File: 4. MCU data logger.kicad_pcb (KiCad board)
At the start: 2 copper layers, 50.2 x 30.3 mm, 29 parts, among them J1 Conn_01x04_Pin, J2 Conn_01x04_Pin, J3 Conn_01x09_Pin, J4 Conn_02x03_Odd_Even, U1 24LC1025, U2 24LC1025, U4 ATMEGA328P-AU, U5 DS1337S_, Y1 32.768 KHz, Y2 16 MHz

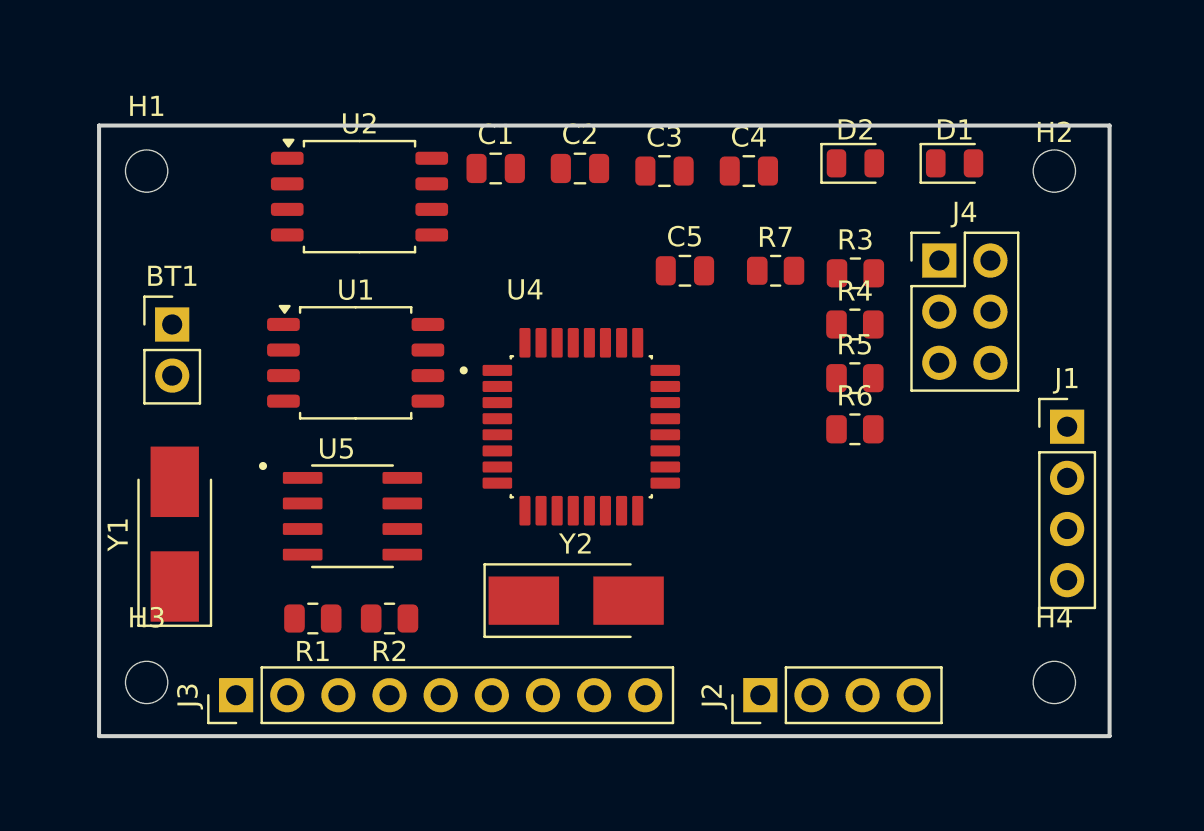
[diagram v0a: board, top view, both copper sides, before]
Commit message: Routing Completed
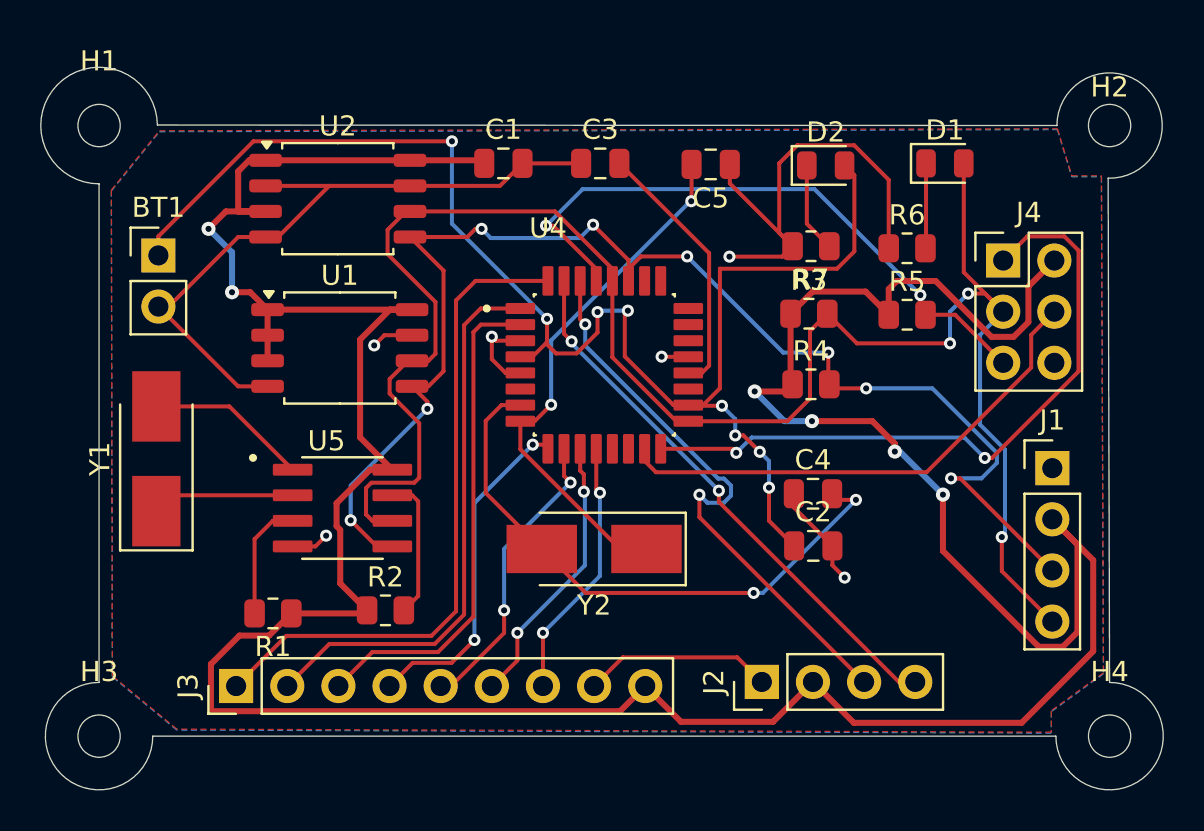
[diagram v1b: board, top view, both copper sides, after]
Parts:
- moved C2 22.0 mm to (80.7, 80.2)
- moved C4 16.3 mm to (80.7, 77.6)
- moved R6 9.36 mm to (85.4, 65.4)
- moved C5 5.44 mm to (75.6, 61.3), turned to 180 degrees
- moved R5 4.08 mm to (85.4, 68.7)
- moved Y1 3.85 mm to (48.1, 75.9)
- moved H4 3.83 mm to (95.5, 89.7)
- moved R4 3.69 mm to (80.6, 72.2)
- moved H3 3.56 mm to (45.3, 89.7)
- moved H2 3.55 mm to (95.5, 59.3)
- moved BT1 3.50 mm to (48.2, 65.8)
- moved U4 3.28 mm to (70.4, 71.2)
- moved H1 3.27 mm to (45.3, 59.3)
- moved C3 3.21 mm to (70.2, 61.2)
- moved J4 3.17 mm to (90.2, 66.0)
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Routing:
- net /VCC: track 0.00 -> 175.4 mm, vias 0 -> 6
- net /SCK: track 0.00 -> 91.7 mm, vias 0 -> 3
- net GND: track 0.00 -> 81.6 mm, vias 0 -> 6
- net Net-(BT1-+): track 0.00 -> 73.0 mm, vias 0 -> 8
- net /SDA: track 0.00 -> 67.7 mm, vias 0 -> 8
- net /MISO: track 0.00 -> 33.9 mm, vias 0 -> 2
- net /D2: track 0.00 -> 32.9 mm
- net /RESET: track 0.00 -> 31.4 mm, vias 0 -> 2
- net Net-(U4-PB6): track 0.00 -> 29.3 mm, vias 0 -> 2
- net /RX: track 0.00 -> 28.5 mm, vias 0 -> 2
- net /D3: track 0.00 -> 27.8 mm
- net /TX: track 0.00 -> 27.6 mm, vias 0 -> 2
- net Net-(U4-PB7): track 0.00 -> 26.4 mm, vias 0 -> 2
- net /MOSI: track 0.00 -> 25.4 mm
- net /D4: track 0.00 -> 24.8 mm
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- added copper zone on F.Cu, net /VCC
- added copper zone on B.Cu, net GND
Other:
- board size 50.2 x 30.3 mm -> 55.8 x 35.9 mm
